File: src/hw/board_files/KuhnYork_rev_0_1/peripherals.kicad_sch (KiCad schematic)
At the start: 27 parts, among them J5 Conn_01x04, J6 Molex 104031-0811, Q1 PMOS, U4 NEO-M9N, U5 SHT30-DIS, U6 BQ27411DRZT-G1A

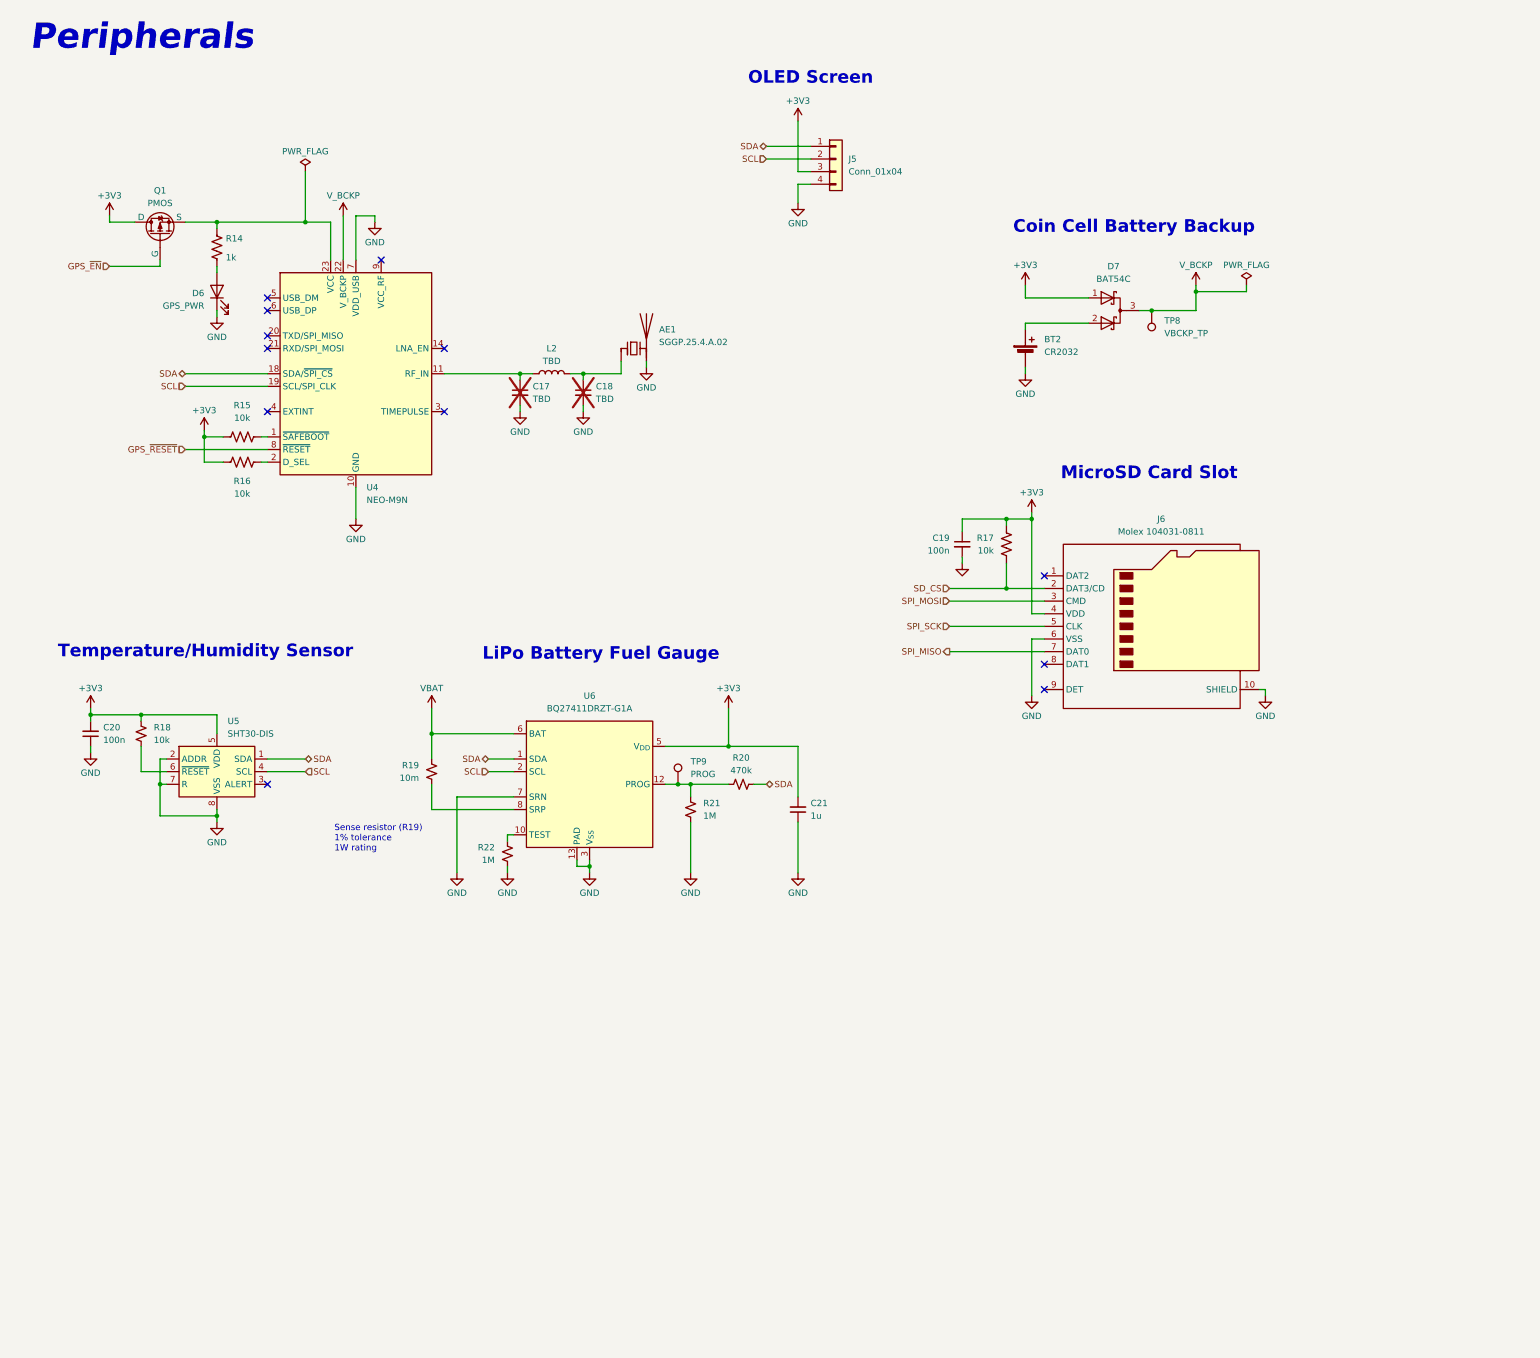
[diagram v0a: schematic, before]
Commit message: rev0.1 done
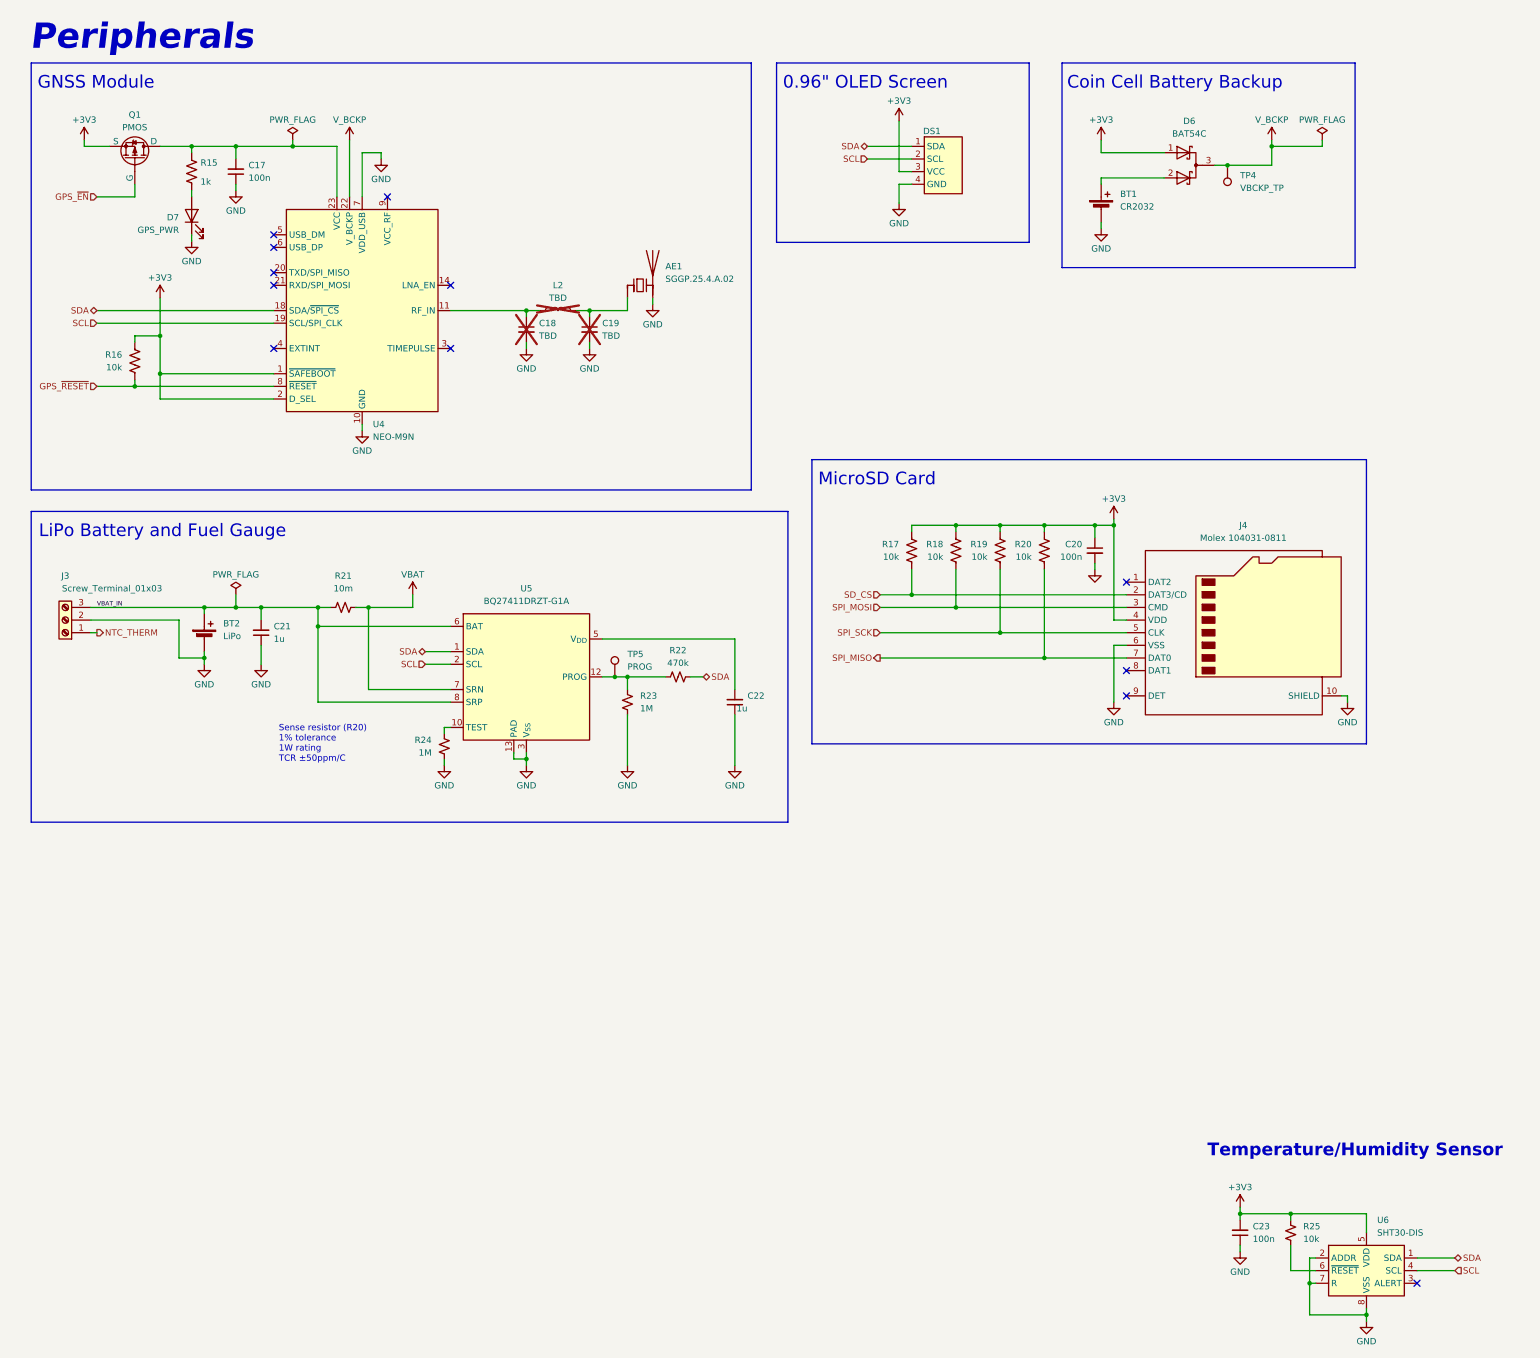
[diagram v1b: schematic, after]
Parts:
- removed J5: Conn_01x04, Connector_PinSocket_2.54mm:PinSocket_1x04_P2.54mm_Vertical, symbol Connector_Generic:Conn_01x04
- removed R15: 10k, Resistor_SMD:R_0603_1608Metric_Pad0.98x0.95mm_HandSolder, symbol Device:R_US
- added BT2: LiPo, Connector_JST:JST_PH_S2B-PH-K_1x02_P2.00mm_Horizontal, symbol Device:Battery_Cell
- added C17: 100n, Capacitor_SMD:C_0603_1608Metric_Pad1.08x0.95mm_HandSolder, symbol Device:C_Small
- added C21: 1u, Capacitor_SMD:C_0603_1608Metric_Pad1.08x0.95mm_HandSolder, symbol Device:C_Small
- added DS1: ~, Project_Library:OLED_128x64_0.96in, symbol Project_Library:OLED_128x64
- added J3: Screw_Terminal_01x03, TerminalBlock_TE-Connectivity:TerminalBlock_TE_282834-3_1x03_P2.54mm_Horizontal, symbol Connector:Screw_Terminal_01x03
- added R18, R19, R20: 10k, Resistor_SMD:R_0603_1608Metric_Pad0.98x0.95mm_HandSolder, symbol Device:R_US
- L2: now not fitted; now left out of the parts list
- TP4: renamed from TP8; footprint TestPoint:TestPoint_Pad_D1.5mm -> TestPoint:TestPoint_Pad_D1.0mm
- TP5: renamed from TP9; footprint TestPoint:TestPoint_Pad_D1.5mm -> TestPoint:TestPoint_Pad_D1.0mm
- renumbered BT2 to BT1, C17 to C18, C18 to C19, C19 to C20, C21 to C22, C20 to C23, D7 to D6, D6 to D7, J6 to J4, R14 to R15, R19 to R21, R20 to R22, R21 to R23, R22 to R24, R18 to R25, U6 to U5, U5 to U6
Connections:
- net +3V3: now also Q1.3 (S), U4.1 (~{SAFEBOOT}), U4.2 (D_SEL), DS1.3 (VCC), R18.1, R19.1, R20.1; no longer C22.2, Q1.1 (D), U5.5 (V_{DD})
- net GND: now also BT2.2 (-), C17.1, C21.1, DS1.4 (GND), DS1.5 (MOUNT), J3.2 (Pin_2); no longer U5.7 (SRN)
- net GPS_~{RESET}: now also R16.2
- net SCL: now also DS1.2 (SCL)
- net SDA: now also DS1.1 (SDA)
- net SPI_MISO: now also R20.2
- net SPI_MOSI: now also R18.2
- net SPI_SCK: now also R19.2
- net VBAT: now also R21.2, U5.7 (SRN); no longer R21.1, U5.6 (BAT)
- net VBAT_IN: now reaches U5.8 (SRP)
- net VBAT_IN: now also R21.1, U5.6 (BAT), BT2.1 (+), C21.2, J3.3 (Pin_3); no longer R21.2
- net at R15.1, U4.23 (VCC): now also Q1.1 (D), C17.2; no longer Q1.3 (S)
- new net: C22.2, U5.5 (V_{DD})
- new net NTC_THERM: J3.1 (Pin_1)
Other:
- note added: "0.96" OLED Screen"
- note added: "GNSS Module"
- note added: "LiPo Battery and Fuel Gauge"
- note added: "MicroSD Card"
- note added: "Sense resistor (R20) 1% tolerance 1W rating TCR ±50ppm/C"
- note removed: "LiPo Battery Fuel Gauge"
- note removed: "MicroSD Card Slot"
- note removed: "OLED Screen"
- note removed: "Sense resistor (R19) 1% tolerance 1W rating"
- moved on the sheet: AE1, BT1, C18, C19, C20, C22, C23, D6, D7, J4, Q1, R15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
